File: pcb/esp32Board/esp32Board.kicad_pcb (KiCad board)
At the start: 4 copper layers, 38.2 x 41.1 mm, 31 parts, among them J1 ESPProgJTAG_RX, J10 USB_C_Receptacle_USB2.0, J2 ESPProg_RX, J3 ESPProgUART_RX, J4 CAN, J5 UART2, J6 I2C, J7 IO, J8 PWR, J9 GND, SW1 SW_Push, U1 ESP32-WROOM-32D, U2 XC6206P332MR

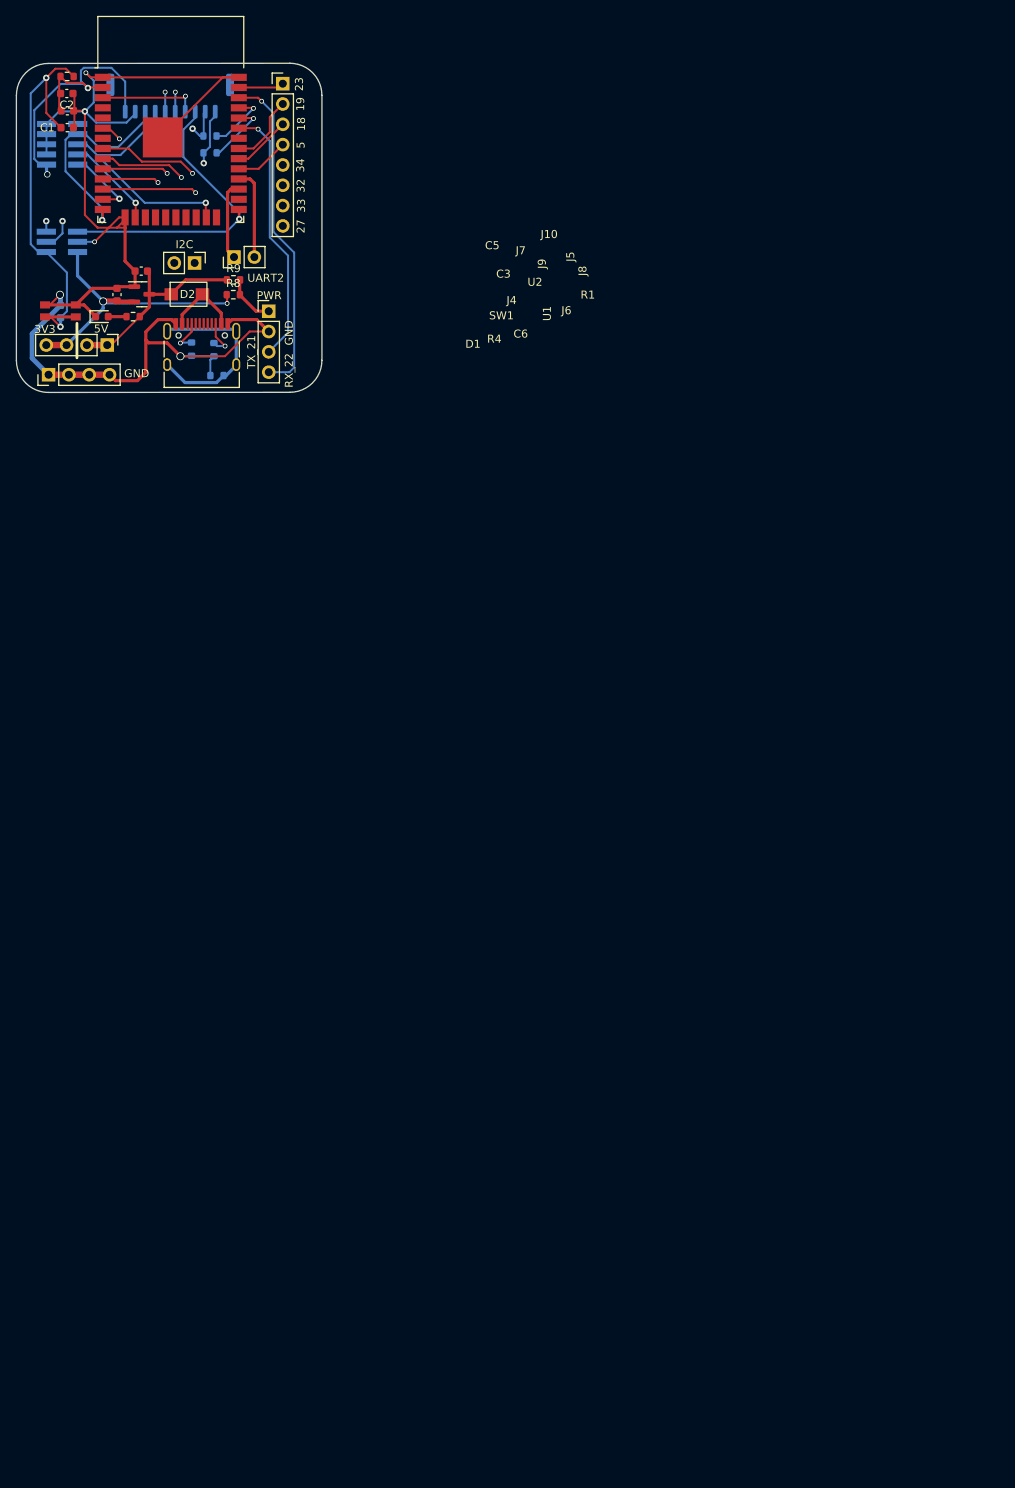
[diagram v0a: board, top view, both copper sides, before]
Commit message: PCB V0.2
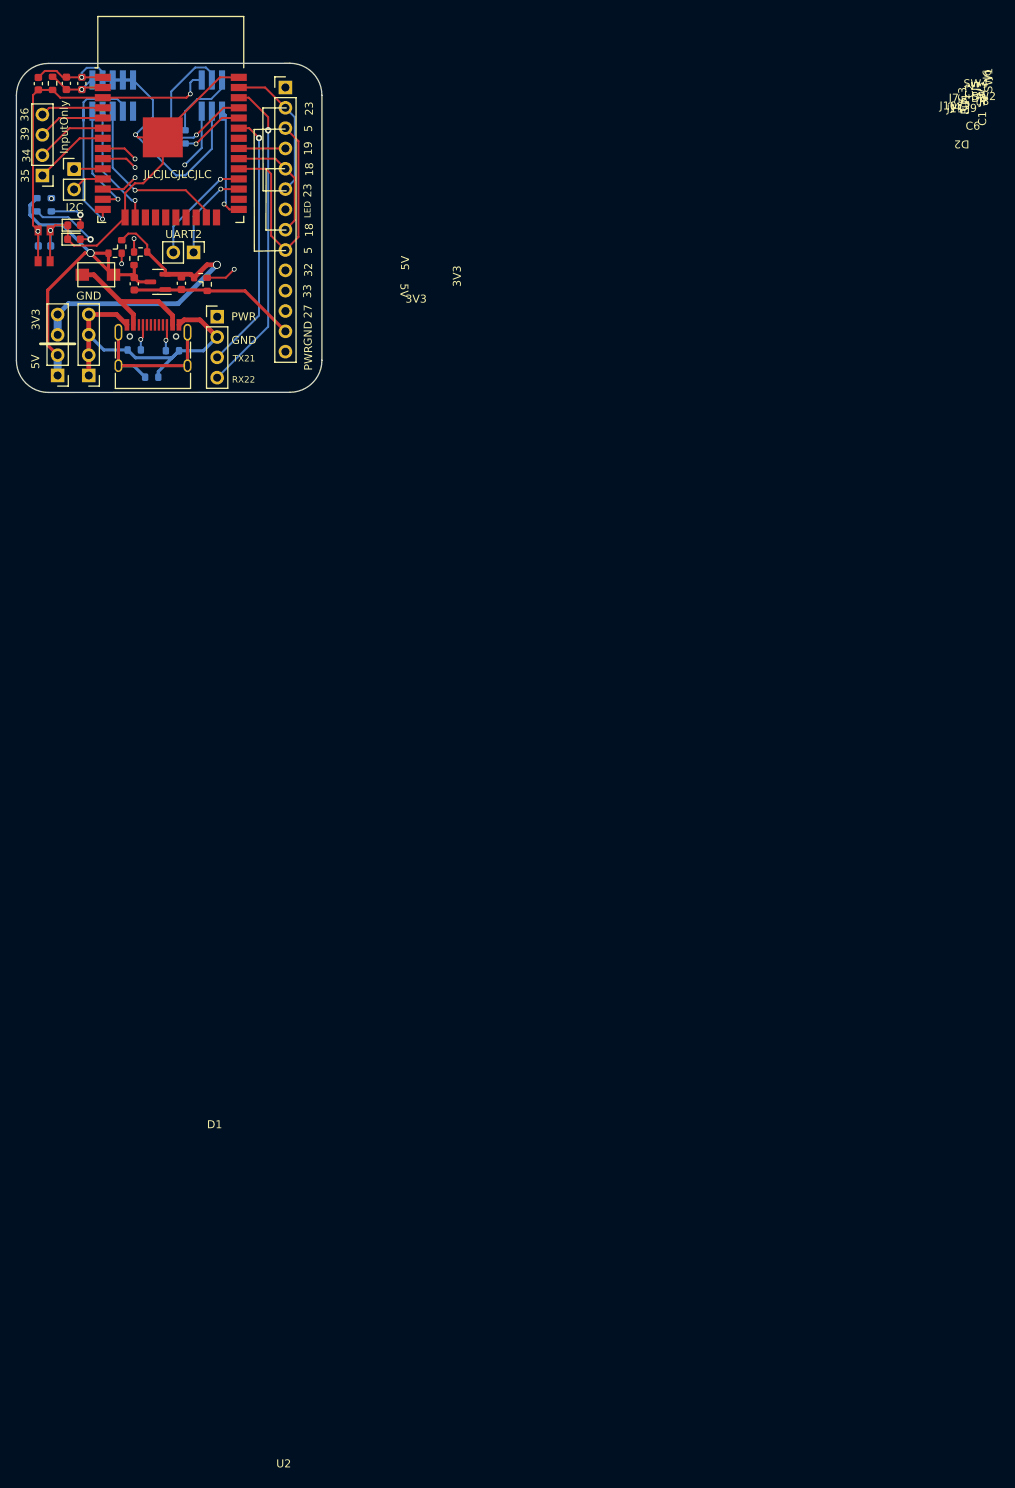
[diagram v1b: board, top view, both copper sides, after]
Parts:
- removed J2: ESPProg_RX, Connector_Molex:Molex_CLIK-Mate_502382-1070_1x10-1MP_P1.25mm_Vertical
- removed R9: 0, Resistor_SMD:R_0603_1608Metric
- added D3: LED, LED_SMD:LED_0603_1608Metric, F.Cu at (146.1, 126.0)
- added J11: Conn_01x14_Female, Connector_PinHeader_2.54mm:PinHeader_1x14_P2.54mm_Vertical, F.Cu at (172.5, 108.8)
- added SW2: SW_Push_SPDT, KisonNew:0603JumperP3, F.Cu at (151.2, 129.5)
- added SW3: SW_Push_SPDT, KisonNew:0603JumperP3, F.Cu at (162.7, 133.4)
- added SW4: SW_Push_SPDT, KisonNew:0603JumperP3, F.Cu at (154.4, 129.3)
- J7: value IO -> InputOnly; footprint Connector_PinHeader_2.54mm:PinHeader_1x08_P2.54mm_Vertical -> Connector_PinHeader_2.54mm:PinHeader_1x04_P2.54mm_Vertical
- R4: value 100k -> 10k; moved to B.Cu
- R8: value 0 -> 10k; moved to B.Cu
- moved J7 32.2 mm to (142.1, 119.8), turned to 180 degrees
- moved J3 26.2 mm to (163.3, 109.8), turned to 180 degrees
- moved R8 25.4 mm to (143.3, 123.4), turned to -90 degrees
- moved J6 19.1 mm to (146.1, 119.0), turned to 0 degrees
- moved R4 18.4 mm to (141.5, 123.4), turned to -90 degrees
- moved D2 11.8 mm to (148.9, 132.2), turned to 180 degrees
- moved D1 10.3 mm to (146.1, 127.7)
- moved SW1 8.89 mm to (142.1, 128.3), turned to -90 degrees
- moved G*** 8.88 mm to (150.0, 131.5), turned to 0 degrees
- moved J1 8.78 mm to (150.9, 109.8), turned to 180 degrees
- moved C4 8.44 mm to (142.4, 128.6), turned to 0 degrees
- moved C6 8.17 mm to (159.5, 133.2), turned to -90 degrees
- moved R5 8.16 mm to (155.8, 145.0), turned to 0 degrees
- moved J8 7.27 mm to (144.0, 144.8), turned to 180 degrees
- moved R6 7.16 mm to (153.6, 141.6), turned to 0 degrees
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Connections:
- J4 pad 1: /CAN_VCC -> Net-(J4-Pad1)
- J7 pad 1: /IO23 -> /IO35
- J7 pad 2: /IO19 -> /IO34
- J7 pad 3: /IO18 -> /IO39
- J7 pad 4: /IO5 -> /IO36
- R8 pad 2: /CAN_VCC -> Net-(D3-Pad2)
- U1 pad 4: unconnected-(U1-Pad4) -> /IO36
- U1 pad 5: unconnected-(U1-Pad5) -> /IO39
- U1 pad 7: unconnected-(U1-Pad7) -> /IO35
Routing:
- net /EN: track 84.0 -> 46.4 mm, vias 3 -> 2
- net Net-(J11-Pad14): track 0.00 -> 26.5 mm, vias 0 -> 1
- net /IO5: track 6.75 -> 32.0 mm
- net /IO0: track 39.0 -> 14.0 mm
- net /RX: track 31.6 -> 9.22 mm, vias 2 -> 0
- net /EXT_5V: track 24.9 -> 46.2 mm, vias 0 -> 1
- net /TX: track 29.9 -> 12.3 mm, vias 2 -> 0
- net /SDA_IO25: track 20.9 -> 3.60 mm, vias 1 -> 0
- net /IO34: track 26.1 -> 8.95 mm, vias 1 -> 0
- net Net-(J4-Pad1): track 0.00 -> 16.0 mm, vias 0 -> 1
- net /TCLK: track 29.9 -> 15.2 mm, vias 2 -> 1
- net Net-(J11-Pad7): track 0.00 -> 13.9 mm, vias 0 -> 1
- net /SCL_IO26: track 18.0 -> 4.13 mm, vias 1 -> 0
- net /TMS: track 27.2 -> 14.2 mm, vias 2 -> 1
- net /IO32: track 24.4 -> 37.0 mm
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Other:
- board text added: "35"
- board text added: "36"
- board text added: "39"
- board text added: "GPPCB-V0.2"
- board text added: "InputOnly"
- board text added: "LED"
- board text added: "RX22"
- board text added: "TX21"
- board text added: "VCC"
- board text added: "屏幕朝向"
- board text removed: "RX_22"
- board text removed: "TX_21"
